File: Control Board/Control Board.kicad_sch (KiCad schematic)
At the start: 43 parts, among them J1 Raspberry_Pi_2_3, J2 Conn_01x03_Pin, J3 Conn_01x03_Pin, J4 Conn_01x03_Pin, J5 Conn_01x03_Pin, J6 Conn_01x03_Pin, J7 Conn_01x03_Pin, J8 Conn_01x04_Pin, Q1 BSS214NH, U1 PIC18F16Q41, U2 PI4ULS5V202UEX

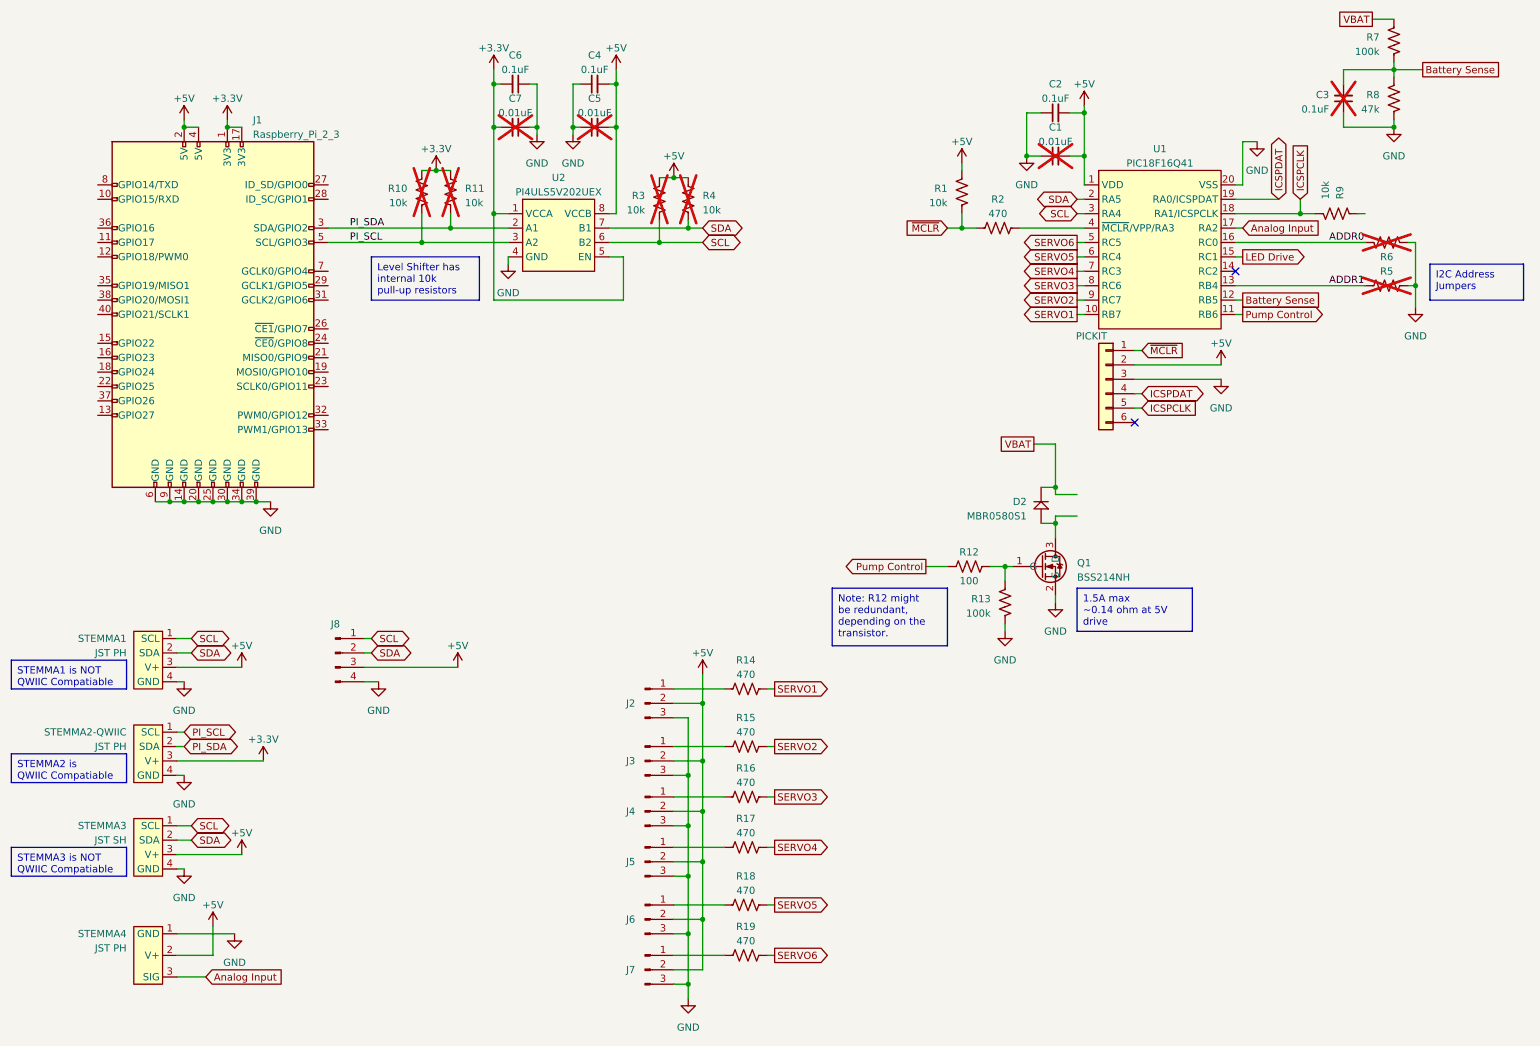
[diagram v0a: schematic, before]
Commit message: Work on Schematic + README
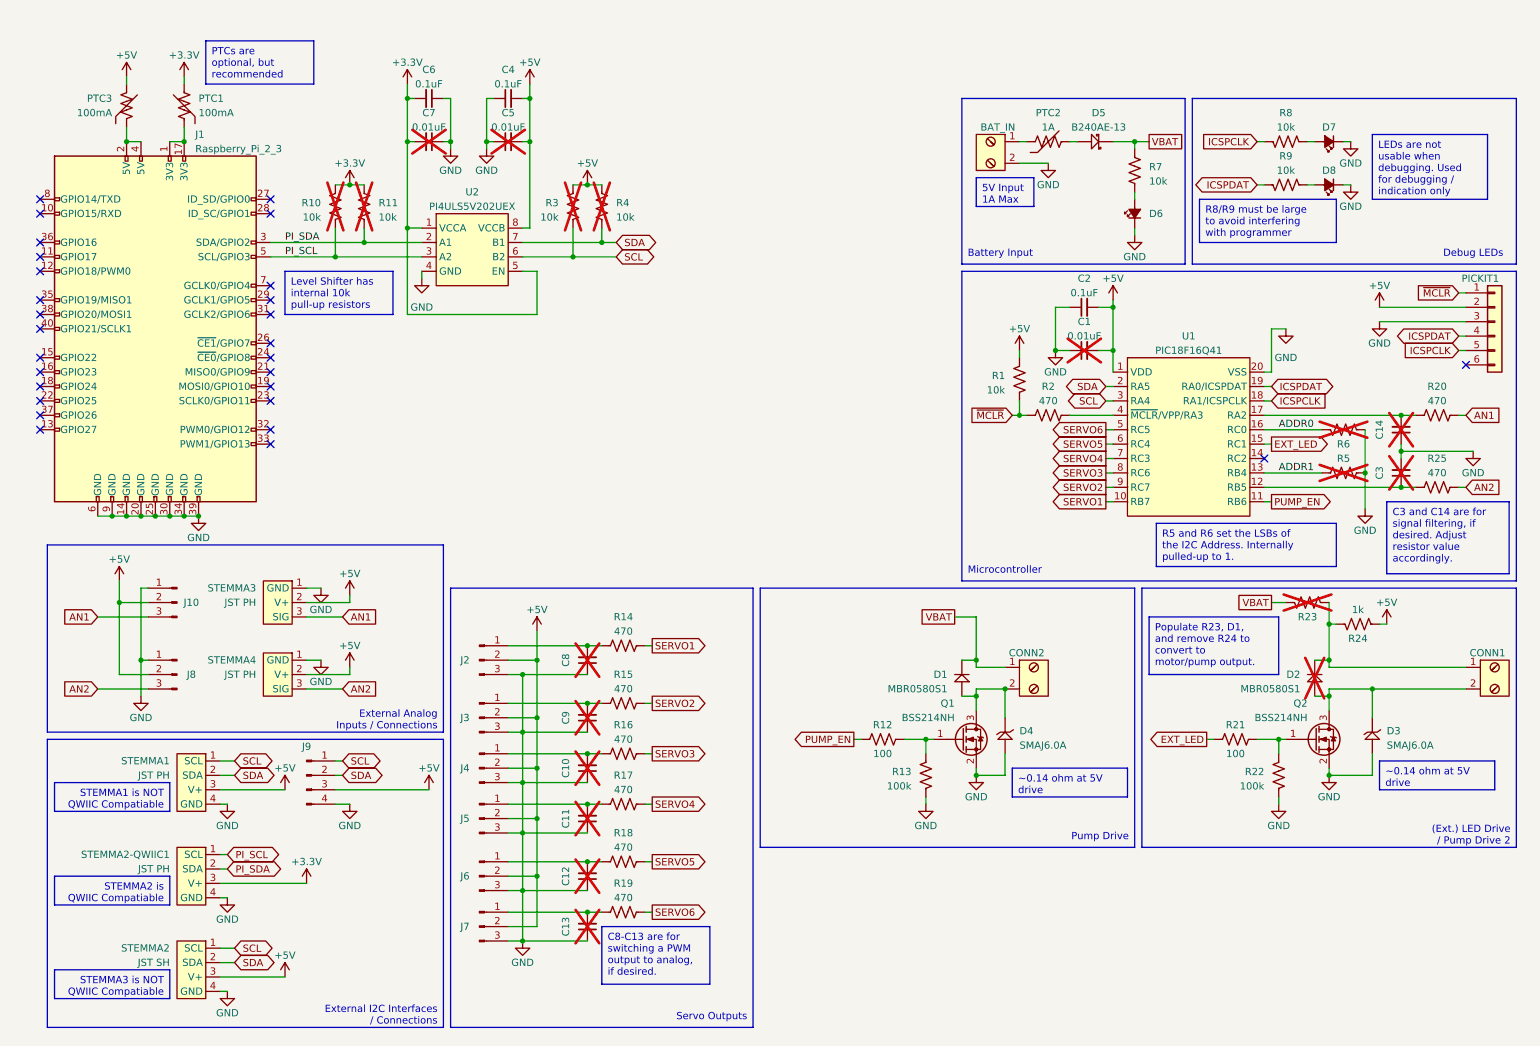
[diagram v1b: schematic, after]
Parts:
- removed J8: Conn_01x04_Pin, symbol Connector:Conn_01x04_Pin
- removed PICKIT: Conn_01x06, symbol Connector_Generic:Conn_01x06
- removed STEMMA2-QWIIC: JST PH, symbol Control Board Parts:STEMMA_4-pin_I2C
- removed STEMMA3: JST SH, symbol Control Board Parts:STEMMA_4-pin_I2C
- added BAT_IN, CONN1, CONN2: ~, symbol Control Board Parts:Terminal_Block
- added C10, C11, C12, C13, C14, C8, C9: 0.01uF, symbol Device:C_Small
- added D2: MBR0580S1, symbol Control Board Parts:MBR0580S1
- added D3, D4: SMAJ6.0A, symbol Control Board Parts:SMAJ
- added D5: B240AE-13, symbol Control Board Parts:Schottky Diode
- added D6, D7, D8: LED_Small_Filled, symbol Device:LED_Small_Filled
- added J10, J8: Conn_01x03_Pin, symbol Connector:Conn_01x03_Pin
- added J9: Conn_01x04_Pin, symbol Connector:Conn_01x04_Pin
- added PICKIT1: Conn_01x06, symbol Connector_Generic:Conn_01x06
- added PTC1, PTC3: 100mA, symbol Control Board Parts:PTC
- added PTC2: 1A, symbol Control Board Parts:PTC
- added Q2: BSS214NH, symbol Control Board Parts:BSS214NH
- added R20, R25: 470, symbol Device:R_US
- added R21: 100, symbol Device:R_US
- added R22: 100k, symbol Device:R_US
- added R23: 0, symbol Device:R_US
- added R24: 1k, symbol Device:R_US
- added STEMMA2: JST SH, symbol Control Board Parts:STEMMA_4-pin_I2C
- added STEMMA2-QWIIC1: JST PH, symbol Control Board Parts:STEMMA_4-pin_I2C
- added STEMMA3: JST PH, symbol Control Board Parts:STEMMA_3-pin_Analog/Digital/PWM
- C3: value 0.1uF -> 0.01uF
- R7: value 100k -> 10k
- R8: value 47k -> 10k
- renumbered D2 to D1
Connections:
- net +3.3V: now also PTC1.2, STEMMA2-QWIIC1.3 (V+); no longer J1.1 (3V3), J1.17 (3V3)
- net +5V: now also J10.2 (Pin_2), J8.2 (Pin_2), J9.3 (Pin_3), PICKIT1.2 (Pin_2), PTC3.2, R24.2, STEMMA2.3 (V+), STEMMA3.2 (V+); no longer J1.2 (5V), J1.4 (5V)
- net GND: now also C3.2, BAT_IN.2, C10.1, C11.1, C12.1, C13.1, C14.1, C8.1, C9.1, D3.a (A), D4.a (A), D6.1 (K), D7.1 (K), D8.1 (K), J10.1 (Pin_1), J8.1 (Pin_1), J9.4 (Pin_4), PICKIT1.3 (Pin_3), Q2.2 (S), R22.2, STEMMA2-QWIIC1.4 (GND), STEMMA2.4 (GND), STEMMA3.1 (GND); no longer C3.1, R8.2
- net ICSPCLK: now also R8.2, PICKIT1.5 (Pin_5); no longer R9.2
- net ICSPDAT: now also R9.2, PICKIT1.4 (Pin_4)
- net PI_SCL: now also STEMMA2-QWIIC1.1 (SCL)
- net PI_SDA: now also STEMMA2-QWIIC1.2 (SDA)
- net SCL: now also J9.1 (Pin_1), STEMMA2.1 (SCL)
- net SDA: now also J9.2 (Pin_2), STEMMA2.2 (SDA)
- net VBAT: now also CONN2.1, D5.K, R23.1
- net ~{MCLR}: now also PICKIT1.1 (Pin_1)
- net at J6.1 (Pin_1), R18.1: now also C12.2
- net at D1.A, Q1.3 (D): now also CONN2.2, D4.K
- net at J7.1 (Pin_1), R19.1: now also C13.2
- net at J5.1 (Pin_1), R17.1: now also C11.2
- net at R9.1: now also D8.2 (A)
- net at J3.1 (Pin_1), R15.1: now also C9.2
- net at J2.1 (Pin_1), R14.1: now also C8.2
- net at J4.1 (Pin_1), R16.1: now also C10.2
- net Analog Input: no longer names the net of U1.17 (RA2)
- net Analog Input: now also C14.2, R20.1; no longer STEMMA4.3 (SIG)
- removed net Battery Sense: C3.2, R7.2, R8.1, U1.12 (RB5)
- net LED Drive renamed EXT_LED
- net EXT_LED: now also R21.1
- net Pump Control renamed PUMP_EN
- new net: D6.2 (A), R7.2
- new net: J1.2 (5V), J1.4 (5V), PTC3.1
- new net: D7.2 (A), R8.1
- new net: CONN1.1, D2.K, R23.2, R24.1
- new net: BAT_IN.1, PTC2.1
- new net: J1.1 (3V3), J1.17 (3V3), PTC1.1
- new net: Q2.1 (G), R21.2, R22.1
- new net: D5.A, PTC2.2
- new net: CONN1.2, D2.A, D3.K, Q2.3 (D)
- new net: C3.1, R25.1, U1.12 (RB5)
- new net AN1: J10.3 (Pin_3), R20.2, STEMMA3.3 (SIG)
- new net AN2: J8.3 (Pin_3), R25.2, STEMMA4.3 (SIG)
- no-connect marks 2 -> 28
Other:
- moved on the sheet: C1, C2, C4, C5, C6, C7, D1, J3, J4, J5, J6, J7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
